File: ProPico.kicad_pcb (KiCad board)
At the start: 2 copper layers, 21 x 51 mm, 56 parts, among them J1 USB_C_Receptacle_USB2.0, J2 SWD, J3 LEFT, J4 RIGHT, SW1 BOOTSEL, SW2 RES, U1 FM24CL16B, U2 W25Q128JVS, U3 TLV1117-33, U4 LM4040DBZ-3, U5 RP2040, Y1 ECS-120-12-36-AGN-TR3

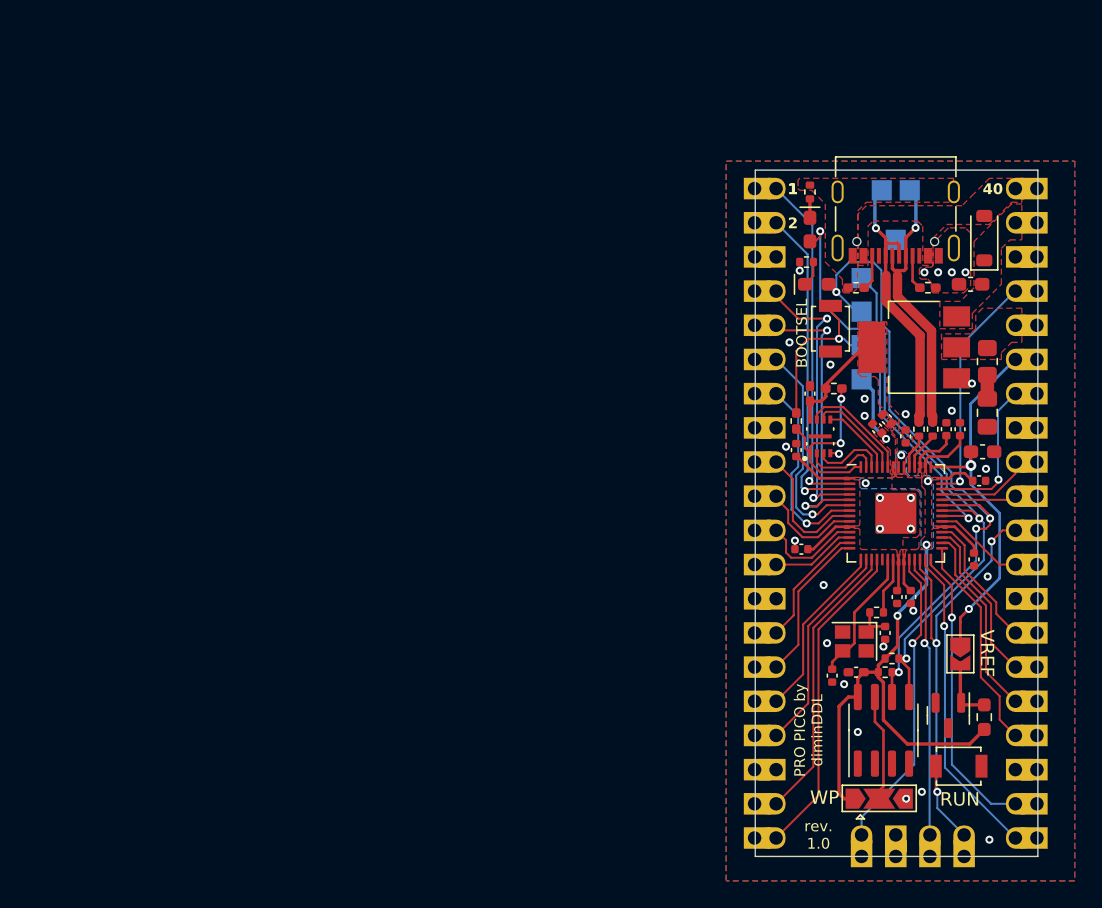
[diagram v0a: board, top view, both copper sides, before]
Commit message: made schematic less cringe
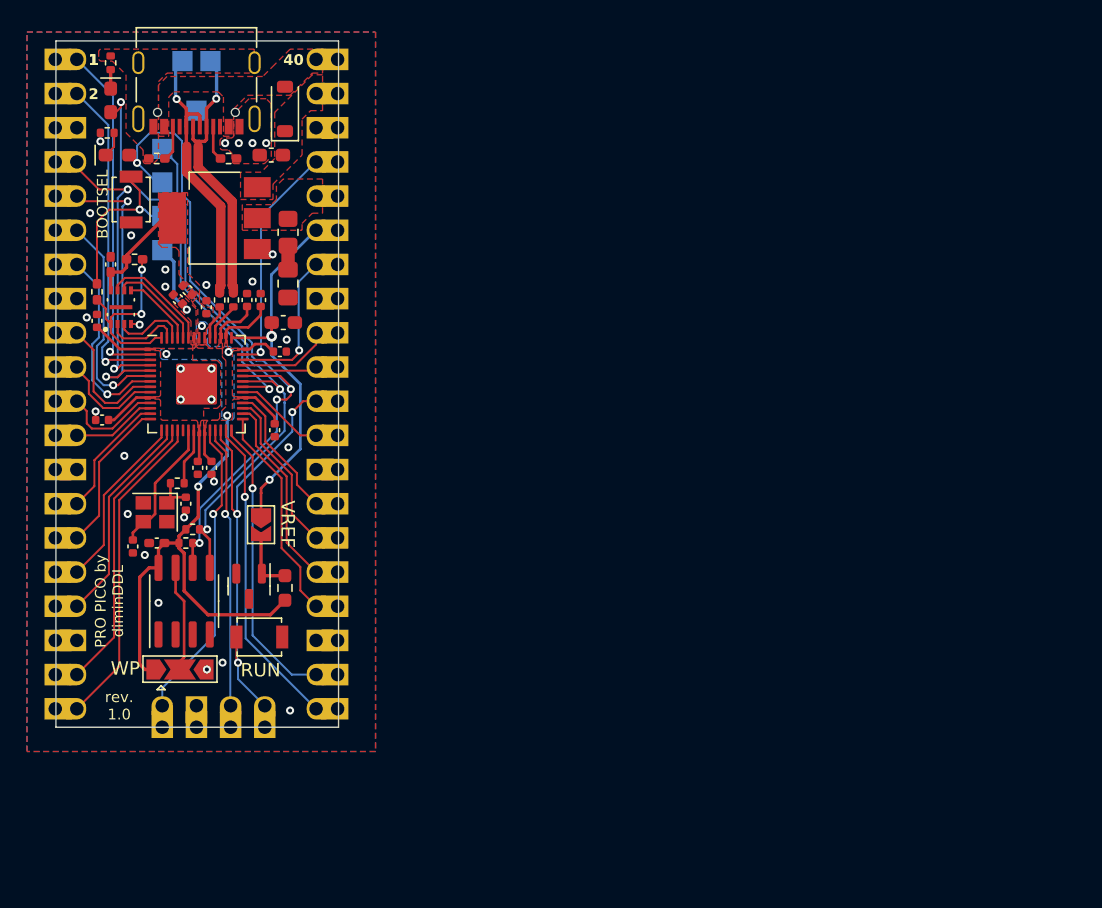
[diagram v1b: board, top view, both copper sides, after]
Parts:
- moved C4 52.8 mm to (108.4, 47.8)
- moved C8 52.8 mm to (101.5, 58.5)
- moved JP2 52.8 mm to (107.7, 75.3)
- moved R2 52.8 mm to (98.3, 55.5)
- moved C1 52.8 mm to (99.9, 76.6)
- moved C10 52.8 mm to (106.6, 58.6)
- moved C11 52.8 mm to (108.7, 68.2)
- moved C14 52.8 mm to (109.1, 62.4)
- moved C15 52.8 mm to (102.2, 57.8)
- moved C16 52.8 mm to (95.5, 60.1)
- moved C17 52.8 mm to (95.9, 67.5)
- moved C18 52.8 mm to (103.0, 71.0)
- moved C2 52.8 mm to (98.1, 76.9)
- moved C6 52.8 mm to (109.7, 57.4)
- moved D1 52.8 mm to (109.4, 44.4)
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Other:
- board text removed: "TODO: check EEPROM pinouts check diode footprint and pins"
